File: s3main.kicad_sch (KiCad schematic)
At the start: 139 parts, among them J1 TRACK, J2 IDC, J3 POWER, J4 USB_C_Receptacle_USB2.0_16P, J5 ZUSI, Q1 QS6K21, Q10 BC847B, Q2 BC847BDW1, Q3 SiS4634LDN, Q4 SiS4634LDN, Q5 SiS4634LDN, Q6 QS6K21, Q7 SiS4634LDN, Q8 SiS4634LDN, Q9 BSS138, SW1 EN, SW2 BOOT, U1 LM393, U10 BTS4141N, U2 7402, U3 TLV9061xDBV, U4 ESP32-S3-WROOM-2, U5 DRV8328B, U6 TPS281C100A, U7 AP63205WU, U8 TXS0102DCT, U9 AZ1117-3.3

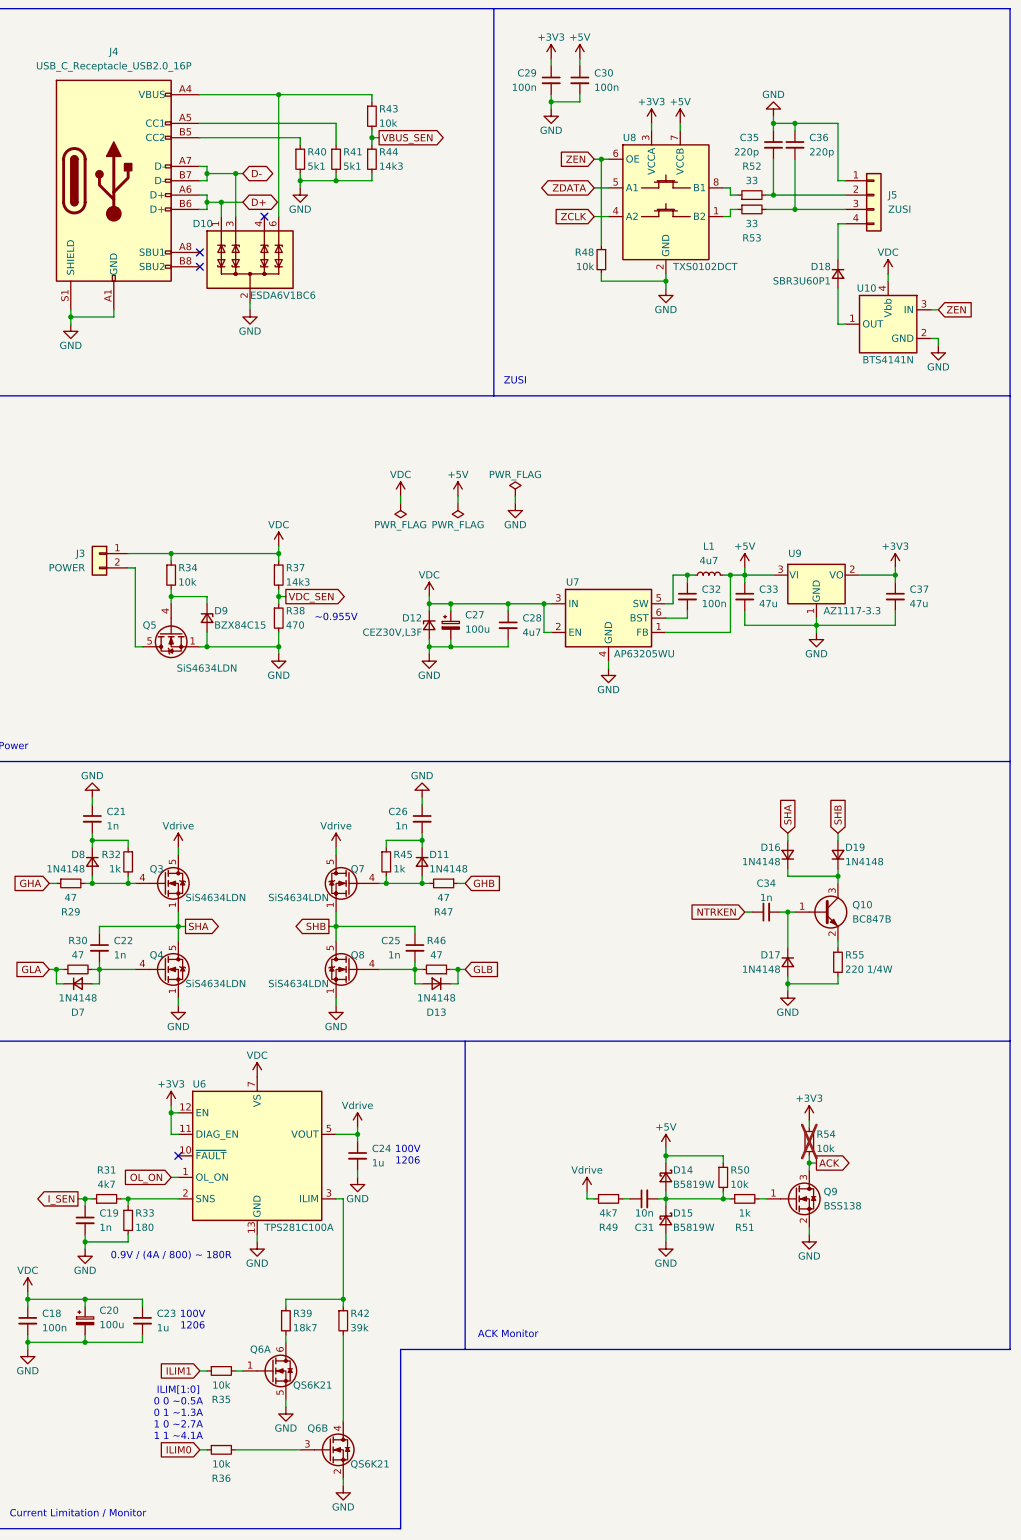
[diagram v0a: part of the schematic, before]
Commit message: chore: replace ACK circuit with TPS281C100 fault pin
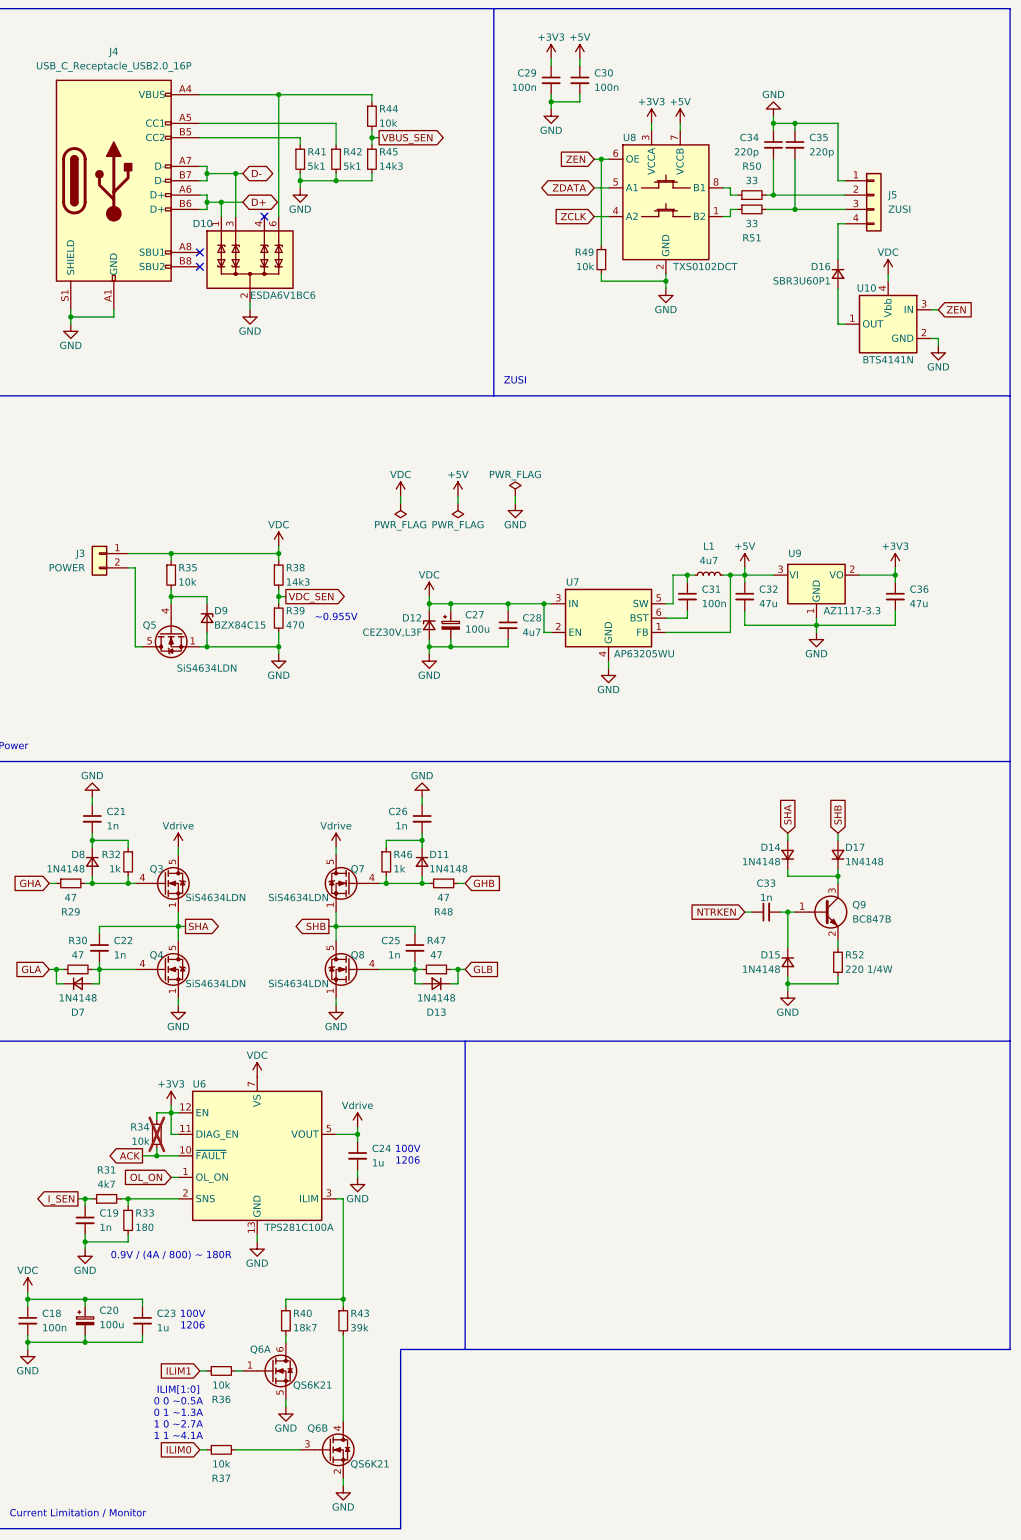
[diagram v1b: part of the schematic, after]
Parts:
- removed C31: 10n, Capacitor_SMD:C_1206_3216Metric, symbol Device:C_Small
- removed D14, D15: B5819W, Diode_SMD:D_SOD-123, symbol Device:D_Schottky_Small
- removed Q9: BSS138, Package_TO_SOT_SMD:TSOT-23, symbol Transistor_FET:Q_NMOS_GSD
- removed R49: 4k7, Resistor_SMD:R_0402_1005Metric, symbol Device:R_Small
- removed R50: 10k, Resistor_SMD:R_0402_1005Metric, symbol Device:R_Small
- removed R51: 1k, Resistor_SMD:R_0402_1005Metric, symbol Device:R_Small
- renumbered C32 to C31, C33 to C32, C34 to C33, C35 to C34, C36 to C35, C37 to C36, D16 to D14, D17 to D15, D18 to D16, D19 to D17, Q10 to Q9, R54 to R34, R34 to R35, R35 to R36, R36 to R37, R37 to R38, R38 to R39, R39 to R40, R40 to R41, R41 to R42, R42 to R43, R43 to R44, R44 to R45, R45 to R46, R46 to R47, R47 to R48, R48 to R49, R52 to R50, R53 to R51, R55 to R52
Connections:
- net ACK: now also U6.10 (~{FAULT})
- no-connect marks 5 -> 4
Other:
- note removed: "ACK Monitor"
- moved on the sheet: R34

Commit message: revert: chore: replace ACK circuit with TPS281C100 fault pin
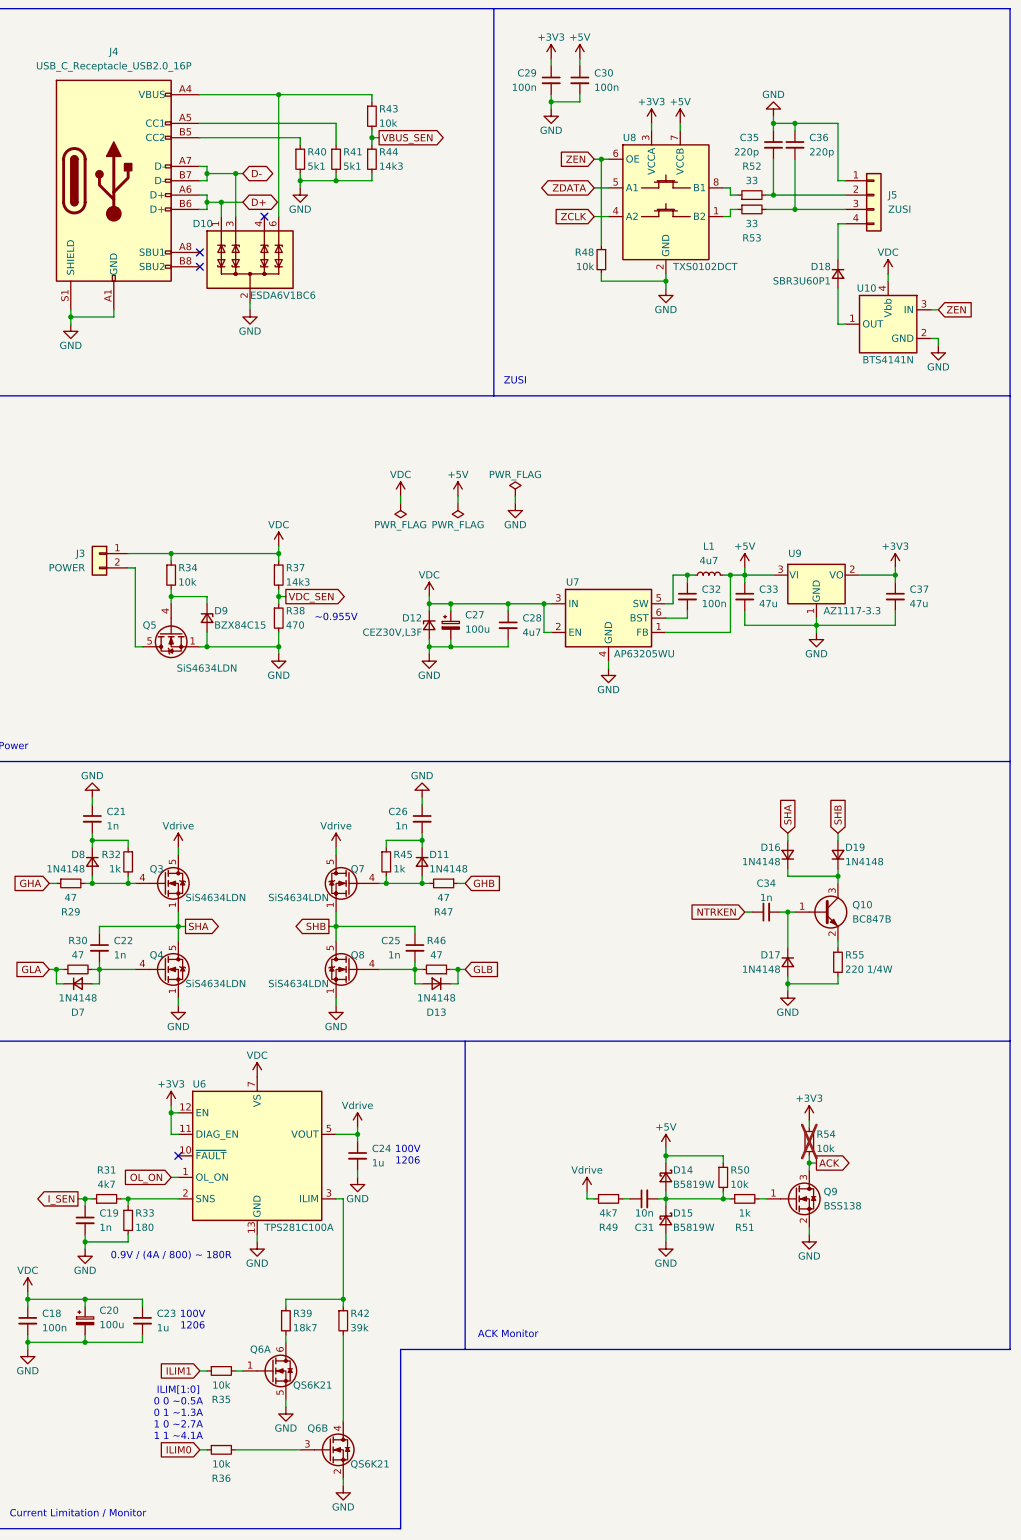
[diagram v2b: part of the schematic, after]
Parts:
- added C31: 10n, Capacitor_SMD:C_1206_3216Metric, symbol Device:C_Small
- added D14, D15: B5819W, Diode_SMD:D_SOD-123, symbol Device:D_Schottky_Small
- added Q9: BSS138, Package_TO_SOT_SMD:TSOT-23, symbol Transistor_FET:Q_NMOS_GSD
- added R49: 4k7, Resistor_SMD:R_0402_1005Metric, symbol Device:R_Small
- added R50: 10k, Resistor_SMD:R_0402_1005Metric, symbol Device:R_Small
- added R51: 1k, Resistor_SMD:R_0402_1005Metric, symbol Device:R_Small
- renumbered C31 to C32, C32 to C33, C33 to C34, C34 to C35, C35 to C36, C36 to C37, D14 to D16, D15 to D17, D16 to D18, D17 to D19, Q9 to Q10, R35 to R34, R36 to R35, R37 to R36, R38 to R37, R39 to R38, R40 to R39, R41 to R40, R42 to R41, R43 to R42, R44 to R43, R45 to R44, R46 to R45, R47 to R46, R48 to R47, R49 to R48, R50 to R52, R51 to R53, R34 to R54, R52 to R55
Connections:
- net +5V: now also D14.1 (K), R50.1
- net ACK: now also Q9.3 (D); no longer U6.10 (~{FAULT})
- net GND: now also D15.2 (A), Q9.2 (S)
- net Vdrive: now also R49.1
- new net: C31.2, D14.2 (A), D15.1 (K), R50.2, R51.1
- new net: C31.1, R49.2
- new net: Q9.1 (G), R51.2
- no-connect marks 4 -> 5
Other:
- note added: "ACK Monitor"
- moved on the sheet: R54
